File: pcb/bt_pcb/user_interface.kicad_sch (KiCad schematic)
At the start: 70 parts, among them J10 AudioJack3_Switch, J11 AudioJack3_Switch, J16 AudioJack3_Switch, J4 Conn_01x10, J9 AudioJack3_Switch, SW1 SW_Push, SW10 RotaryEncoder_Switch, SW2 SW_Push, SW3 SW_Push, SW4 SW_Push, SW5 SW_Push, SW6 SW_Push, SW7 SW_Push, SW8 SW_Push, SW9 SW_Push

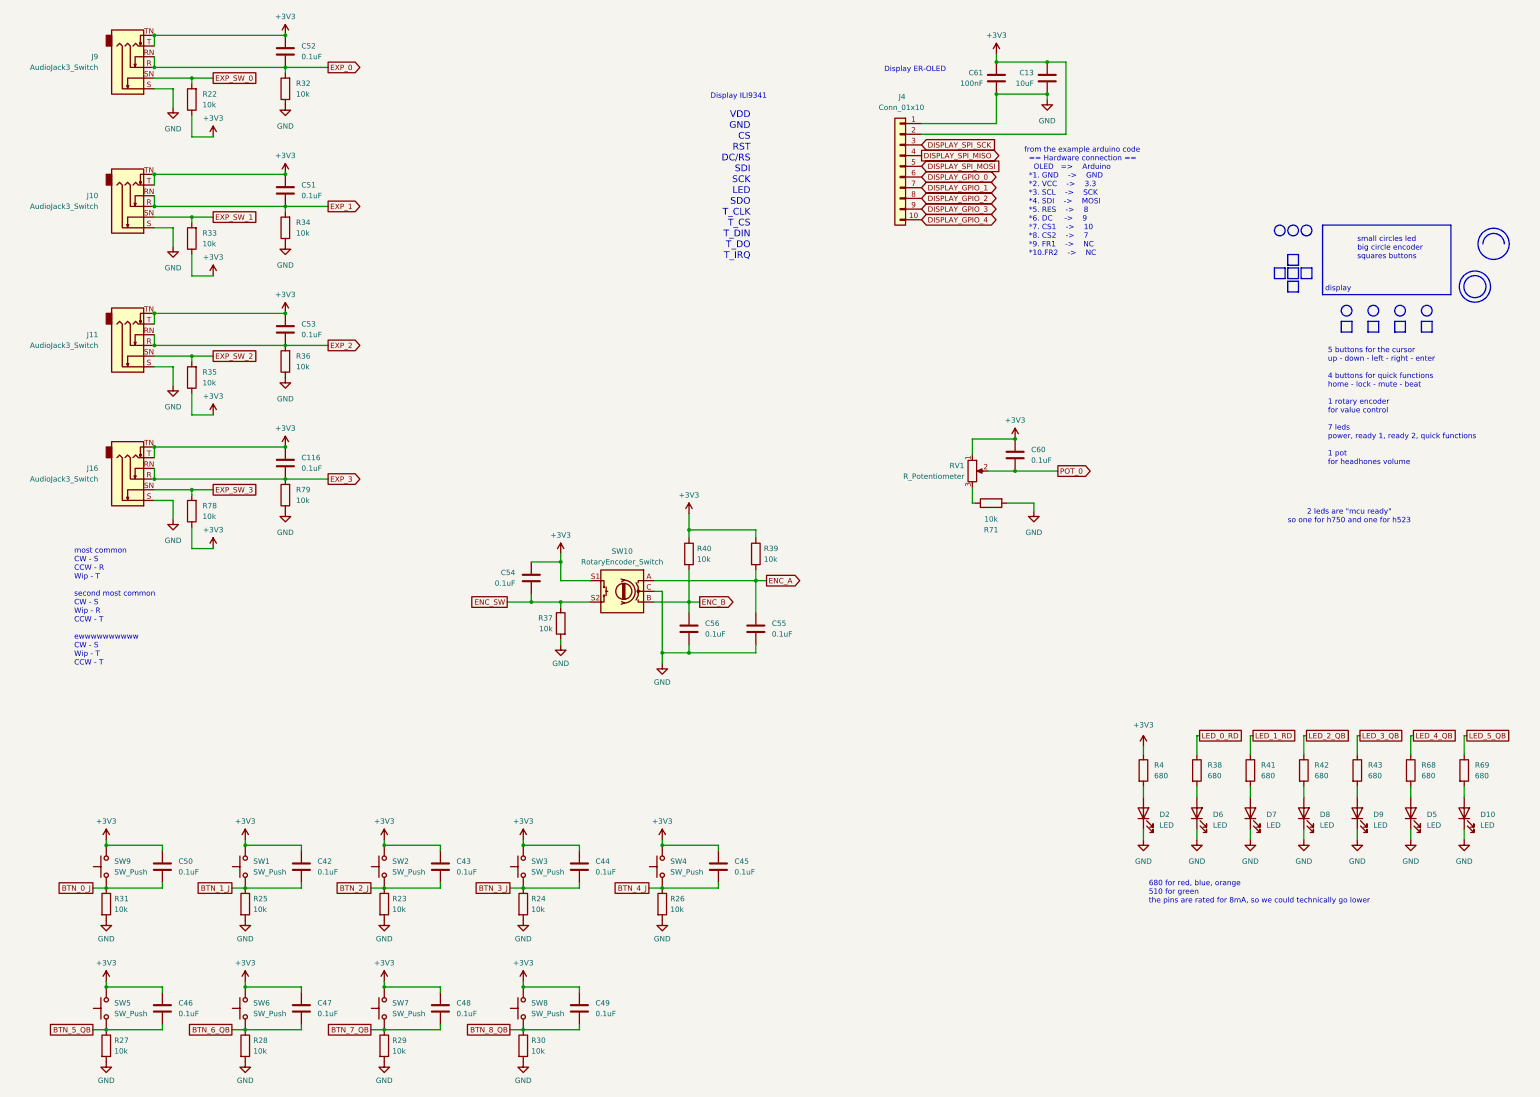
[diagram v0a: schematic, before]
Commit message: solving some erc warnings and errors
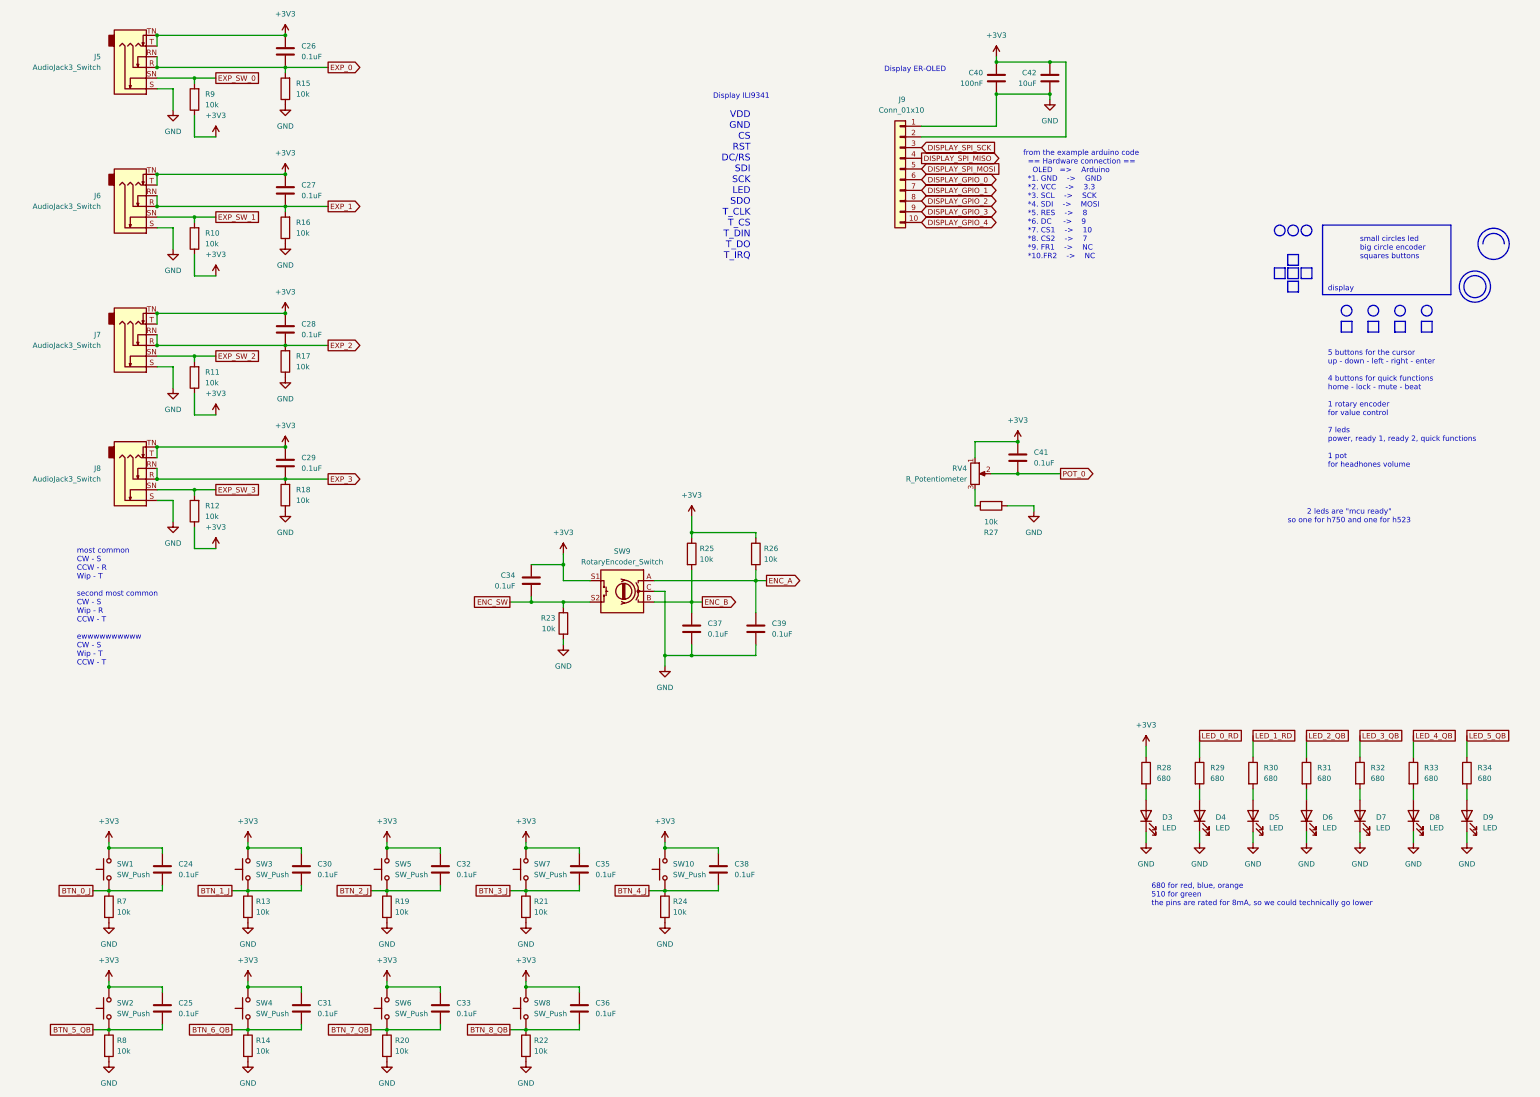
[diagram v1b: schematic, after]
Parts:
- removed D10, D2: LED, symbol Device:LED
- added D3, D4: LED, symbol Device:LED
- renumbered C50 to C24, C46 to C25, C52 to C26, C51 to C27, C53 to C28, C116 to C29, C42 to C30, C47 to C31, C43 to C32, C48 to C33, C54 to C34, C44 to C35, C49 to C36, C56 to C37, C45 to C38, C55 to C39, C61 to C40, C60 to C41, C13 to C42, J9 to J5, J10 to J6, J11 to J7, J16 to J8, J4 to J9, R33 to R10, R35 to R11, R78 to R12, R25 to R13, R28 to R14, R32 to R15, R34 to R16, R36 to R17, R79 to R18, R23 to R19, R29 to R20, R24 to R21, R30 to R22, R37 to R23, R26 to R24, R40 to R25, R39 to R26, R71 to R27, R4 to R28, R38 to R29, R41 to R30, R42 to R31, R43 to R32, R68 to R33, R69 to R34, R31 to R7, R27 to R8, R22 to R9, RV1 to RV4, SW9 to SW1, SW4 to SW10, SW5 to SW2, SW1 to SW3, SW6 to SW4, SW2 to SW5, SW7 to SW6, SW3 to SW7, SW10 to SW9
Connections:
- net GND: now also D3.1 (K), D4.1 (K)
- net at R30.2: now also D5.2 (A); no longer D7.2 (A)
- net at R31.2: now also D6.2 (A); no longer D8.2 (A)
- net at R34.2: now also D9.2 (A)
- net at R32.2: now also D7.2 (A); no longer D9.2 (A)
- net at R28.2: now also D3.2 (A)
- net at R33.2: now also D8.2 (A); no longer D5.2 (A)
- net at R29.2: now also D4.2 (A); no longer D6.2 (A)
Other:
- moved on the sheet: C24, C30, C32, C34, C35, C37, C38, C41, C42, J5, J6, J7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
